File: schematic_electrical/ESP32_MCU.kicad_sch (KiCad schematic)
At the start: 14 parts, among them U1 ESP32_S2_PICO

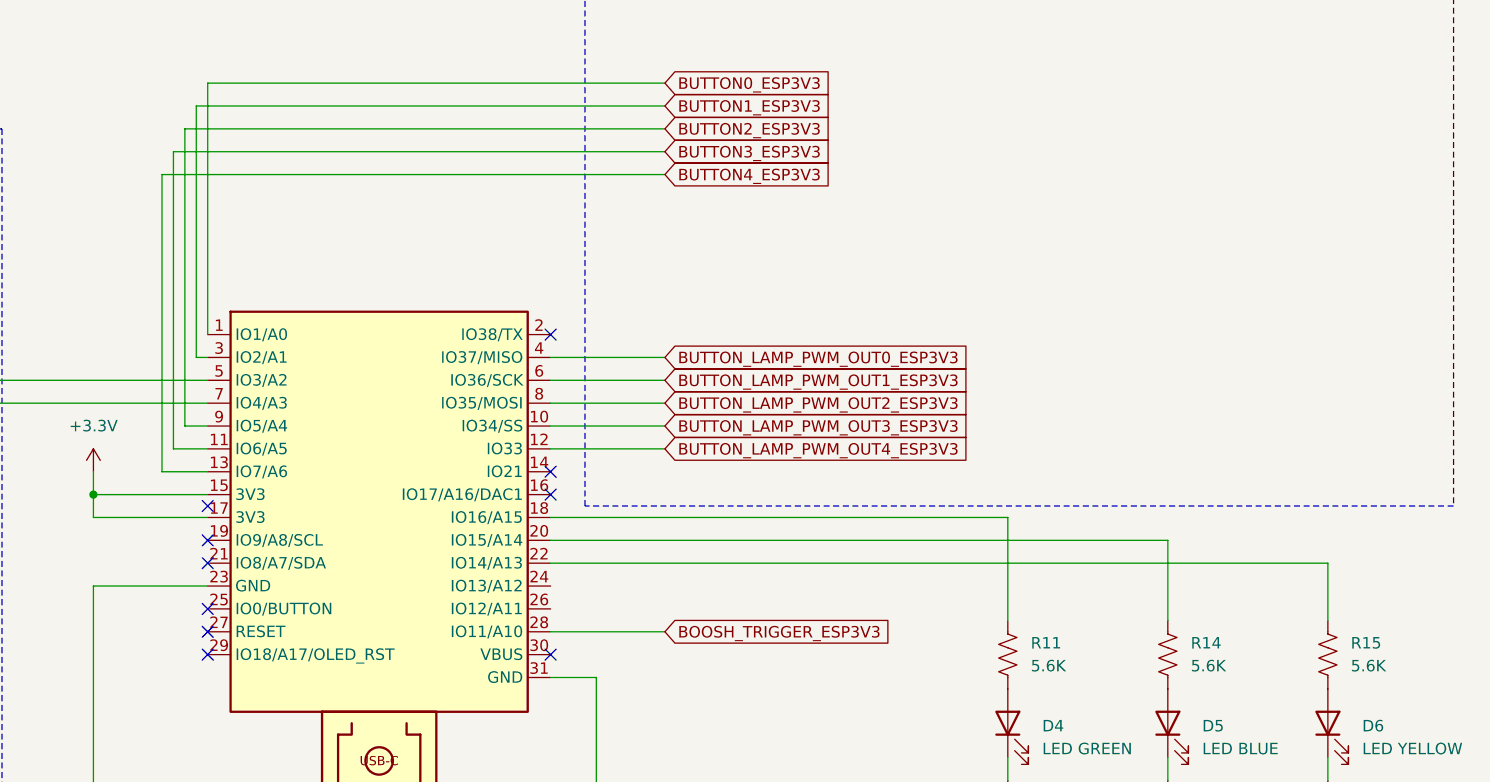
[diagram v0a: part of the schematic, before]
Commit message: delete button4
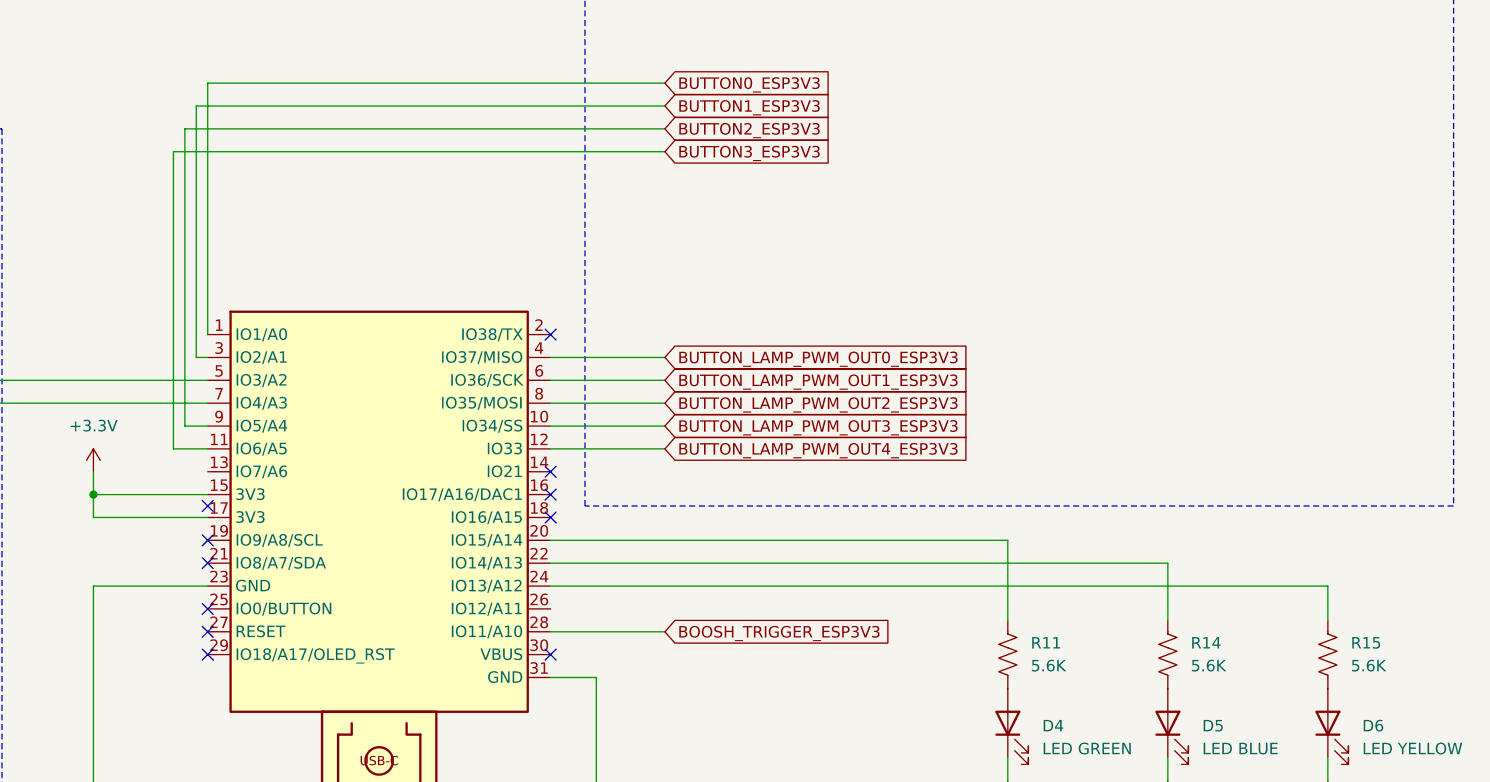
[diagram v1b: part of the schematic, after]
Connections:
- net at U1.18 (IO16/A15): no longer R11.2
- net at U1.20 (IO15/A14): now also R11.2; no longer R14.2
- net at U1.22 (IO14/A13): now also R14.2; no longer R15.2
- net at U1.24 (IO13/A12): now also R15.2
- net BUTTON4_ESP3V3: no longer names the net of U1.13 (IO7/A6)
- no-connect marks 10 -> 11
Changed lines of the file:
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@@
+	)
+	(no_connect
+		(at 180.34 81.28)
 	)
 	(no_connect
@@
 	(wire
 		(pts
-			(xy 266.7 86.36) (xy 266.7 92.71)
-		)
-		(stroke
-			(width 0)
-			(type default)
-		)
-	)
-	(wire
-		(pts
 			(xy 266.7 107.95) (xy 266.7 110.49)
 		)
@@
 	(wire
 		(pts
+			(xy 180.34 88.9) (xy 266.7 88.9)
+		)
+		(stroke
+			(width 0)
+			(type default)
+		)
+	)
+	(wire
+		(pts
 			(xy 161.29 119.38) (xy 161.29 146.05)
 		)
@@
 	(wire
 		(pts
-			(xy 180.34 81.28) (xy 231.14 81.28)
-		)
-		(stroke
-			(width 0)
-			(type default)
-		)
-	)
-	(wire
-		(pts
 			(xy 82.55 63.5) (xy 82.55 60.96)
 		)
@@
 	(wire
 		(pts
-			(xy 231.14 81.28) (xy 231.14 92.71)
+			(xy 180.34 83.82) (xy 231.14 83.82)
 		)
 		(stroke
@@
 	(wire
 		(pts
+			(xy 231.14 83.82) (xy 231.14 92.71)
+		)
+		(stroke
+			(width 0)
+			(type default)
+		)
+	)
+	(wire
+		(pts
 			(xy 180.34 99.06) (xy 185.42 99.06)
 		)
@@
 	(wire
 		(pts
-			(xy 180.34 83.82) (xy 248.92 83.82)
-		)
-		(stroke
-			(width 0)
-			(type default)
-		)
-	)
-	(wire
-		(pts
 			(xy 80.01 118.11) (xy 80.01 115.57)
 		)
@@
 	(wire
 		(pts
-			(xy 248.92 83.82) (xy 248.92 92.71)
-		)
-		(stroke
-			(width 0)
-			(type default)
-		)
-	)
-	(wire
-		(pts
 			(xy 140.97 63.5) (xy 142.24 63.5)
 		)
@@
 	(wire
 		(pts
-			(xy 137.16 76.2) (xy 142.24 76.2)
+			(xy 266.7 88.9) (xy 266.7 92.71)
 		)
 		(stroke
@@
 	(wire
 		(pts
-			(xy 137.16 43.18) (xy 193.04 43.18)
+			(xy 180.34 86.36) (xy 248.92 86.36)
 		)
 		(stroke
@@
 	(wire
 		(pts
-			(xy 180.34 86.36) (xy 266.7 86.36)
-		)
-		(stroke
-			(width 0)
-			(type default)
-		)
-	)
-	(wire
-		(pts
 			(xy 129.54 78.74) (xy 129.54 76.2)
 		)
@@
 	(wire
 		(pts
+			(xy 248.92 86.36) (xy 248.92 92.71)
+		)
+		(stroke
+			(width 0)
+			(type default)
+		)
+	)
+	(wire
+		(pts
 			(xy 161.29 146.05) (xy 176.53 146.05)
 		)
@@
 		(pts
 			(xy 63.5 125.73) (xy 63.5 127)
-		)
-		(stroke
-			(width 0)
-			(type default)
-		)
-	)
-	(wire
-		(pts
-			(xy 137.16 43.18) (xy 137.16 76.2)
 		)
 		(stroke
@@
 			(effects
 				(font
-					(size 1.27 1.27)
-				)
-				(justify left)
-				(hide yes)
-			)
-		)
-	)
-	(global_label "BUTTON4_ESP3V3"
-		(shape input)
-		(at 193.04 43.18 0)
-		(fields_autoplaced yes)
-		(effects
-			(font
-				(size 1.27 1.27)
-			)
-			(justify left)
-		)
-		(property "Intersheetrefs" "${INTERSHEET_REFS}"
-			(at 204.4314 43.18 0)
-			(effects
-				(font
